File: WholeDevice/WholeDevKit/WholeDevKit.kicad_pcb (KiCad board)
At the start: 2 copper layers, 4 parts

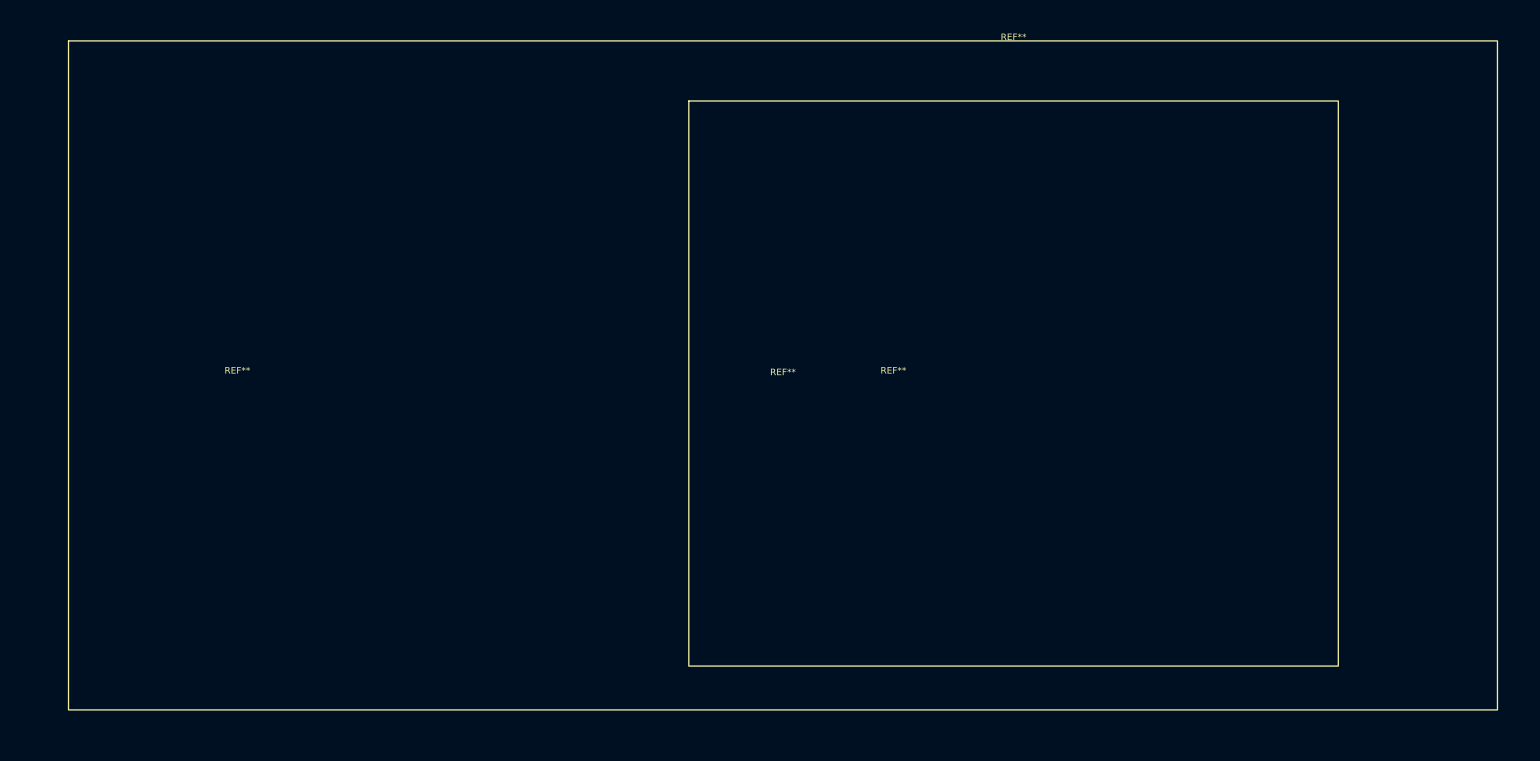
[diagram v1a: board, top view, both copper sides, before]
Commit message: movedconnectors
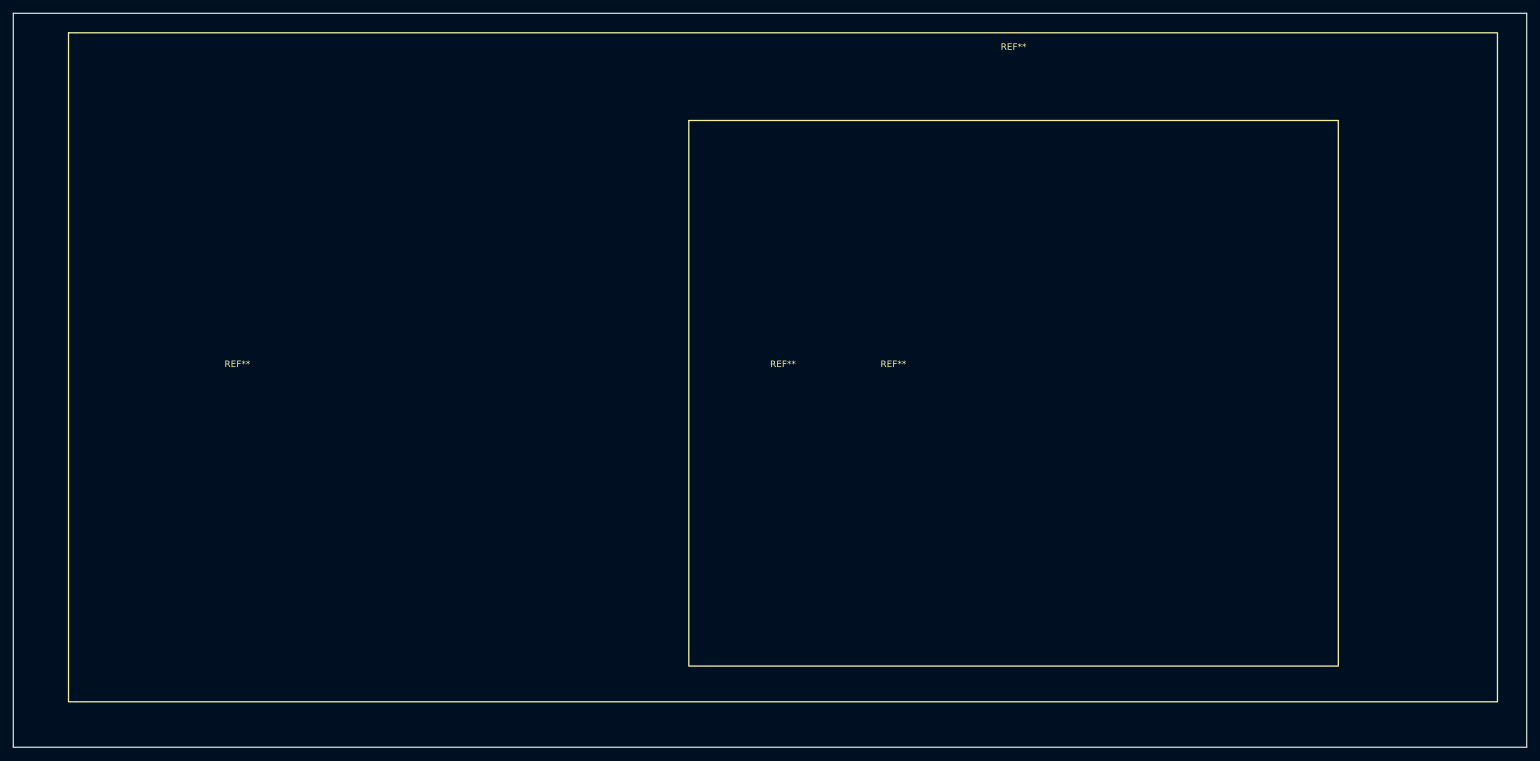
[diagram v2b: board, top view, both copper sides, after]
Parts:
- removed the REF** at (156.0, 81.5)
- removed the REF** at (36.5, 80.0)
- added REF**: LogicBoard-DevKit, GigaVescLibs:LogicBoard-DevKit, F.Cu at (156.0, 83.0)
- added REF**: PowerBoard-LT8316, GigaVescLibs:PowerBoard-LT8316, F.Cu at (36.5, 79.0)
- moved REF** 1.25 mm to (120.5, 79.0)
- moved REF** 1.00 mm to (137.5, 79.0)
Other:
- board outline added: 233 x 113 mm
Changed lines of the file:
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@@
   )
   (net 0 "")
-  (footprint "GigaVescLibs:LogicBoard" (layer "F.Cu")
-    (at 156 81.5)
-    (attr smd)
-    (fp_text reference "REF**" (at 0 -53.34 unlocked) (layer "F.SilkS")
-        (effects (font (size 1 1) (thickness 0.1)))
-    )
-    (fp_text value "LogicBoard" (at 0 1 unlocked) (layer "F.Fab")
-        (effects (font (size 1 1) (thickness 0.15)))
-    )
-    (fp_text user "${REFERENCE}" (at 0 2.5 unlocked) (layer "F.Fab")
-        (effects (font (size 1 1) (thickness 0.15)))
-    )
-    (fp_rect (start -50 -43.5) (end 50 43.5)
-      (stroke (width 0.1) (type default)) (fill none) (layer "F.SilkS"))
-    (model "A:/Projects/Electronic/GigaESC/LogicBoard/DevKit/DevKit.wrl"
-      (offset (xyz 0 0 21))
-      (scale (xyz 1 1 1))
-      (rotate (xyz 0 0 0))
-    )
-  )
   (footprint "GigaVescLibs:MosfetBoardIXTT220N20X4HV" (layer "F.Cu")
-    (at 137.5 80)
+    (at 137.5 79)
     (attr smd)
     (fp_text reference "REF**" (at 0 -0.5 unlocked) (layer "F.SilkS")
@@
     )
   )
-  (footprint "GigaVescLibs:PowerBoard" (layer "F.Cu")
-    (at 36.5 80)
+  (footprint "GigaVescLibs:LogicBoard-DevKit" (layer "F.Cu")
+    (at 156 83)
+    (attr smd)
+    (fp_text reference "REF**" (at 0 -53.34 unlocked) (layer "F.SilkS")
+        (effects (font (size 1 1) (thickness 0.1)))
+    )
+    (fp_text value "LogicBoard-DevKit" (at 0 1 unlocked) (layer "F.Fab")
+        (effects (font (size 1 1) (thickness 0.15)))
+    )
+    (fp_text user "${REFERENCE}" (at 0 2.5 unlocked) (layer "F.Fab")
+        (effects (font (size 1 1) (thickness 0.15)))
+    )
+    (fp_rect (start -50 -42) (end 50 42)
+      (stroke (width 0.1) (type default)) (fill none) (layer "F.SilkS"))
+    (model "A:/Projects/Electronic/GigaESC/LogicBoard/DevKit/DevKit.wrl"
+      (offset (xyz 0 0 21))
+      (scale (xyz 1 1 1))
+      (rotate (xyz 0 0 0))
+    )
+  )
+  (footprint "GigaVescLibs:PowerBoard-LT8316" (layer "F.Cu")
+    (at 36.5 79)
     (attr through_hole)
     (fp_text reference "REF**" (at 0 -0.5 unlocked) (layer "F.SilkS")
         (effects (font (size 1 1) (thickness 0.1)))
     )
-    (fp_text value "PowerBoard" (at 0 1 unlocked) (layer "F.Fab")
+    (fp_text value "PowerBoard-LT8316" (at 0 1 unlocked) (layer "F.Fab")
         (effects (font (size 1 1) (thickness 0.15)))
     )
@@
       (stroke (width 0.05) (type default)) (fill none) (layer "F.CrtYd"))
     (model "A:/Projects/Electronic/GigaESC/PowerBoard/LT8316/LT8316.wrl"
-      (offset (xyz 0 0 9))
+      (offset (xyz 0 0 8))
       (scale (xyz 1 1 1))
       (rotate (xyz 0 0 0))
@@
   )
   (footprint "GigaVescLibs:Hammond1455N2202" (layer "F.Cu")
-    (at 120.5 80.25)
+    (at 120.5 79)
     (attr smd)
     (fp_text reference "REF**" (at 0 -0.5 unlocked) (layer "F.SilkS")
@@
     )
   )
+  (gr_rect (start 2 24.5) (end 235 137.5)
+    (stroke (width 0.1) (type default)) (fill none) (layer "Edge.Cuts"))
 )
